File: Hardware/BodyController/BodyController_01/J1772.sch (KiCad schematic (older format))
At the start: 14 parts, among them Q3 2N7002

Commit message: New bring-up code for Body Controller
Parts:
- D9: MPN PMEG10010ELRX -> PMEG6020AELRX
- R177: value 340k -> 560k; MPN ERJ-3EKF3403V -> AC0603FR-07560KL
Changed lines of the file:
@@
 F 1 "D_Schottky" H 2650 1500 50  0000 C CNN
 F 2 "Diodes_SMD:D_SOD-123" H 2650 1600 50  0001 C CNN
-F 3 "https://assets.nexperia.com/documents/data-sheet/PMEG10010ELR.pdf" H 2650 1600 50  0001 C CNN
-F 4 "PMEG10010ELRX" H 2650 1800 50  0001 C CNN "MPN"
+F 3 "https://assets.nexperia.com/documents/data-sheet/PMEG6020AELR.pdf" H 2650 1600 50  0001 C CNN
+F 4 "PMEG6020AELRX" H 2650 1800 50  0001 C CNN "MPN"
 F 5 "y" H 2650 1800 50  0001 C CNN "populate"
 	1    2650 1600
@@
 P 4500 1850
 F 0 "R177" V 4580 1850 50  0000 C CNN
-F 1 "340k" V 4500 1850 50  0000 C CNN
+F 1 "560k" V 4500 1850 50  0000 C CNN
 F 2 "Resistors_SMD:R_0603" V 4430 1850 50  0001 C CNN
-F 3 "https://industrial.panasonic.com/cdbs/www-data/pdf/RDA0000/AOA0000C304.pdf" H 4500 1850 50  0001 C CNN
-F 4 "ERJ-3EKF3403V" H 4580 1950 50  0001 C CNN "MPN"
+F 3 "http://www.yageo.com/NewPortal/yageodocoutput?fileName=/pdf/R-Chip/PYu-AC_51_RoHS_L_6.pdf" H 4500 1850 50  0001 C CNN
+F 4 "AC0603FR-07560KL" H 4580 1950 50  0001 C CNN "MPN"
 F 5 "y" H 4580 1950 50  0001 C CNN "populate"
 	1    4500 1850
@@
 	0    1    1    0
 $EndComp
+$Comp
+L C C138
+U 1 1 5A63943B
+P 2050 1850
+F 0 "C138" H 2075 1950 50  0000 L CNN
+F 1 "10nF" H 2075 1750 50  0000 L CNN
+F 2 "Capacitors_SMD:C_0603" H 2088 1700 50  0001 C CNN
+F 3 "https://product.tdk.com/info/en/documents/chara_sheet/CGA3E2X7R1H103K080AA.pdf" H 2050 1850 50  0001 C CNN
+F 4 "CGA3E2X7R1H103K080AA" H 2075 2050 50  0001 C CNN "MPN"
+F 5 "y" H 2075 2050 50  0001 C CNN "populate"
+	1    2050 1850
+	1    0    0    -1
+$EndComp
+$Comp
+L GND #PWR0284
+U 1 1 5A639442
+P 2050 2050
+F 0 "#PWR0284" H 2050 1800 50  0001 C CNN
+F 1 "GND" H 2050 1900 50  0000 C CNN
+F 2 "" H 2050 2050 50  0001 C CNN
+F 3 "" H 2050 2050 50  0001 C CNN
+	1    2050 2050
+	1    0    0    -1
+$EndComp
+$Comp
+L C C139
+U 1 1 5A6394A0
+P 3650 4650
+F 0 "C139" H 3675 4750 50  0000 L CNN
+F 1 "10nF" H 3675 4550 50  0000 L CNN
+F 2 "Capacitors_SMD:C_0603" H 3688 4500 50  0001 C CNN
+F 3 "https://product.tdk.com/info/en/documents/chara_sheet/CGA3E2X7R1H103K080AA.pdf" H 3650 4650 50  0001 C CNN
+F 4 "CGA3E2X7R1H103K080AA" H 3675 4850 50  0001 C CNN "MPN"
+F 5 "y" H 3675 4850 50  0001 C CNN "populate"
+	1    3650 4650
+	1    0    0    -1
+$EndComp
+$Comp
+L GND #PWR0285
+U 1 1 5A6394A7
+P 3650 4850
+F 0 "#PWR0285" H 3650 4600 50  0001 C CNN
+F 1 "GND" H 3650 4700 50  0000 C CNN
+F 2 "" H 3650 4850 50  0001 C CNN
+F 3 "" H 3650 4850 50  0001 C CNN
+	1    3650 4850
+	1    0    0    -1
+$EndComp
 Text GLabel 1750 1600 0    60   Input ~ 0
 PILOT
@@
 Wire Wire Line
 	3300 4300 4500 4300
+Wire Wire Line
+	2050 2050 2050 2000
+Wire Wire Line
+	3650 4850 3650 4800
+Wire Wire Line
+	2050 1700 2050 1600
+Wire Wire Line
+	3650 4500 3650 4300
 Connection ~ 3200 1600
 Connection ~ 3800 1600
@@
 Connection ~ 5550 4350
 Connection ~ 4500 4300
-$Comp
-L C C138
-U 1 1 5A63943B
-P 2050 1850
-F 0 "C138" H 2075 1950 50  0000 L CNN
-F 1 "10nF" H 2075 1750 50  0000 L CNN
-F 2 "Capacitors_SMD:C_0603" H 2088 1700 50  0001 C CNN
-F 3 "https://product.tdk.com/info/en/documents/chara_sheet/CGA3E2X7R1H103K080AA.pdf" H 2050 1850 50  0001 C CNN
-F 4 "CGA3E2X7R1H103K080AA" H 2075 2050 50  0001 C CNN "MPN"
-F 5 "y" H 2075 2050 50  0001 C CNN "populate"
-	1    2050 1850
-	1    0    0    -1
-$EndComp
-$Comp
-L GND #PWR0284
-U 1 1 5A639442
-P 2050 2050
-F 0 "#PWR0284" H 2050 1800 50  0001 C CNN
-F 1 "GND" H 2050 1900 50  0000 C CNN
-F 2 "" H 2050 2050 50  0001 C CNN
-F 3 "" H 2050 2050 50  0001 C CNN
-	1    2050 2050
-	1    0    0    -1
-$EndComp
-Wire Wire Line
-	2050 2050 2050 2000
-$Comp
-L C C139
-U 1 1 5A6394A0
-P 3650 4650
-F 0 "C139" H 3675 4750 50  0000 L CNN
-F 1 "10nF" H 3675 4550 50  0000 L CNN
-F 2 "Capacitors_SMD:C_0603" H 3688 4500 50  0001 C CNN
-F 3 "https://product.tdk.com/info/en/documents/chara_sheet/CGA3E2X7R1H103K080AA.pdf" H 3650 4650 50  0001 C CNN
-F 4 "CGA3E2X7R1H103K080AA" H 3675 4850 50  0001 C CNN "MPN"
-F 5 "y" H 3675 4850 50  0001 C CNN "populate"
-	1    3650 4650
-	1    0    0    -1
-$EndComp
-$Comp
-L GND #PWR0285
-U 1 1 5A6394A7
-P 3650 4850
-F 0 "#PWR0285" H 3650 4600 50  0001 C CNN
-F 1 "GND" H 3650 4700 50  0000 C CNN
-F 2 "" H 3650 4850 50  0001 C CNN
-F 3 "" H 3650 4850 50  0001 C CNN
-	1    3650 4850
-	1    0    0    -1
-$EndComp
-Wire Wire Line
-	3650 4850 3650 4800
-Wire Wire Line
-	2050 1700 2050 1600
 Connection ~ 2050 1600
-Wire Wire Line
-	3650 4500 3650 4300
 Connection ~ 3650 4300
 $EndSCHEMATC

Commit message: too much work to specify all. New Scheduler, new bootloader, added new Hardware projects, updated code for bringup, COnverted kicad files to new version.
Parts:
- C131, C132, C138, C139: symbol C -> BodyController_01-rescue:C-RESCUE-BodyController_01
- D9: symbol D_Schottky -> BodyController_01-rescue:D_Schottky-RESCUE-BodyController_01
- Q3: symbol 2N7002 -> BodyController_01-rescue:2N7002-RESCUE-BodyController_01
- R176, R177, R178, R179, R180, R181, R73, R82: symbol R -> BodyController_01-rescue:R-RESCUE-BodyController_01
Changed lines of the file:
@@
-EESchema Schematic File Version 2
-LIBS:switches
-LIBS:power
-LIBS:device
-LIBS:transistors
-LIBS:conn
-LIBS:linear
-LIBS:regul
-LIBS:74xx
-LIBS:cmos4000
-LIBS:adc-dac
-LIBS:memory
-LIBS:xilinx
-LIBS:microcontrollers
-LIBS:dsp
-LIBS:microchip
-LIBS:analog_switches
-LIBS:motorola
-LIBS:texas
-LIBS:intel
-LIBS:audio
-LIBS:interface
-LIBS:digital-audio
-LIBS:philips
-LIBS:display
-LIBS:cypress
-LIBS:siliconi
-LIBS:opto
-LIBS:atmel
-LIBS:contrib
-LIBS:valves
-LIBS:HSD
-LIBS:micros
-LIBS:ICs
-LIBS:Connectors
-LIBS:microchip_dspic33dsc
+EESchema Schematic File Version 4
 LIBS:BodyController_01-cache
-EELAYER 25 0
+EELAYER 26 0
 EELAYER END
 $Descr A4 11693 8268
@@
 $EndDescr
 $Comp
-L D_Schottky D9
+L BodyController_01-rescue:D_Schottky-RESCUE-BodyController_01 D9
 U 1 1 5A54F2A1
 P 2650 1600
@@
 $EndComp
 $Comp
-L R R73
+L BodyController_01-rescue:R-RESCUE-BodyController_01 R73
 U 1 1 5A54F30A
 P 3200 1950
@@
 $EndComp
 $Comp
-L R R176
+L BodyController_01-rescue:R-RESCUE-BodyController_01 R176
 U 1 1 5A54F35D
 P 3800 1950
@@
 $EndComp
 $Comp
-L R R177
+L BodyController_01-rescue:R-RESCUE-BodyController_01 R177
 U 1 1 5A54F390
 P 4500 1850
@@
 $EndComp
 $Comp
-L R R178
+L BodyController_01-rescue:R-RESCUE-BodyController_01 R178
 U 1 1 5A54F3DC
 P 4500 2250
@@
 $EndComp
 $Comp
-L GND #PWR0279
+L BodyController_01-rescue:GND-RESCUE-BodyController_01 #PWR0279
 U 1 1 5A54F42F
 P 4500 2550
@@
 $EndComp
 $Comp
-L GND #PWR0280
+L BodyController_01-rescue:GND-RESCUE-BodyController_01 #PWR0280
 U 1 1 5A54F450
 P 3200 2250
@@
 $EndComp
 $Comp
-L C C131
+L BodyController_01-rescue:C-RESCUE-BodyController_01 C131
 U 1 1 5A54F538
 P 4900 2250
@@
 $EndComp
 $Comp
-L 2N7002 Q3
+L BodyController_01-rescue:2N7002-RESCUE-BodyController_01 Q3
 U 1 1 5A54FBF6
 P 3700 2700
@@
 $EndComp
 $Comp
-L GND #PWR0281
+L BodyController_01-rescue:GND-RESCUE-BodyController_01 #PWR0281
 U 1 1 5A54FC4E
 P 3800 3000
@@
 $EndComp
 $Comp
-L R R82
+L BodyController_01-rescue:R-RESCUE-BodyController_01 R82
 U 1 1 5A54FC87
 P 3250 2700
@@
 $EndComp
 $Comp
-L R R179
+L BodyController_01-rescue:R-RESCUE-BodyController_01 R179
 U 1 1 5A54FFEC
 P 4500 4050
@@
 $EndComp
 $Comp
-L R R180
+L BodyController_01-rescue:R-RESCUE-BodyController_01 R180
 U 1 1 5A54FFF2
 P 4500 4550
@@
 $EndComp
 $Comp
-L GND #PWR0282
+L BodyController_01-rescue:GND-RESCUE-BodyController_01 #PWR0282
 U 1 1 5A54FFF8
 P 4500 4850
@@
 $EndComp
 $Comp
-L C C132
+L BodyController_01-rescue:C-RESCUE-BodyController_01 C132
 U 1 1 5A550002
 P 5550 4550
@@
 $EndComp
 $Comp
-L +5VP #PWR0283
+L BodyController_01-rescue:+5VP-RESCUE-BodyController_01 #PWR0283
 U 1 1 5A5505E6
 P 4500 3800
@@
 $EndComp
 $Comp
-L R R181
+L BodyController_01-rescue:R-RESCUE-BodyController_01 R181
 U 1 1 5A5506C3
 P 5150 4350
@@
 $EndComp
 $Comp
-L C C138
+L BodyController_01-rescue:C-RESCUE-BodyController_01 C138
 U 1 1 5A63943B
 P 2050 1850
@@
 $EndComp
 $Comp
-L GND #PWR0284
+L BodyController_01-rescue:GND-RESCUE-BodyController_01 #PWR0284
 U 1 1 5A639442
 P 2050 2050
@@
 $EndComp
 $Comp
-L C C139
+L BodyController_01-rescue:C-RESCUE-BodyController_01 C139
 U 1 1 5A6394A0
 P 3650 4650
@@
 $EndComp
 $Comp
-L GND #PWR0285
+L BodyController_01-rescue:GND-RESCUE-BodyController_01 #PWR0285
 U 1 1 5A6394A7
 P 3650 4850

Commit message: changed some directory locations, added new DCDC PBC project, few Body controller light and switches changes
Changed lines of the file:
@@
 PROXIMITY
 Wire Wire Line
-	2800 1600 4500 1600
+	2800 1600 3200 1600
 Wire Wire Line
 	3200 1600 3200 1800
@@
 	4500 1600 4500 1700
 Wire Wire Line
-	4500 2000 4500 2100
+	4500 2000 4500 2050
 Wire Wire Line
-	4500 2400 4500 2550
+	4500 2400 4500 2450
 Wire Wire Line
 	4900 2100 4900 2050
 Wire Wire Line
-	4500 2050 5150 2050
+	4500 2050 4900 2050
 Wire Wire Line
 	4500 2450 4900 2450
@@
 	3500 2700 3400 2700
 Wire Wire Line
-	1750 1600 2500 1600
+	1750 1600 2050 1600
 Wire Wire Line
 	3100 2700 2900 2700
@@
 	4500 3800 4500 3900
 Wire Wire Line
-	4500 4200 4500 4400
+	4500 4200 4500 4300
 Wire Wire Line
-	4500 4700 4500 4850
+	4500 4700 4500 4750
 Wire Wire Line
 	5550 4400 5550 4350
 Wire Wire Line
-	5300 4350 5800 4350
+	5300 4350 5550 4350
 Wire Wire Line
 	4500 4750 5550 4750
@@
 	5000 4350 4500 4350
 Wire Wire Line
-	3300 4300 4500 4300
+	3300 4300 3650 4300
 Wire Wire Line
 	2050 2050 2050 2000
@@
 Connection ~ 2050 1600
 Connection ~ 3650 4300
+Wire Wire Line
+	3200 1600 3800 1600
+Wire Wire Line
+	3800 1600 4500 1600
+Wire Wire Line
+	4500 2050 4500 2100
+Wire Wire Line
+	4500 2450 4500 2550
+Wire Wire Line
+	4900 2050 5150 2050
+Wire Wire Line
+	4500 4350 4500 4400
+Wire Wire Line
+	4500 4750 4500 4850
+Wire Wire Line
+	5550 4350 5800 4350
+Wire Wire Line
+	4500 4300 4500 4350
+Wire Wire Line
+	2050 1600 2500 1600
+Wire Wire Line
+	3650 4300 4500 4300
 $EndSCHEMATC

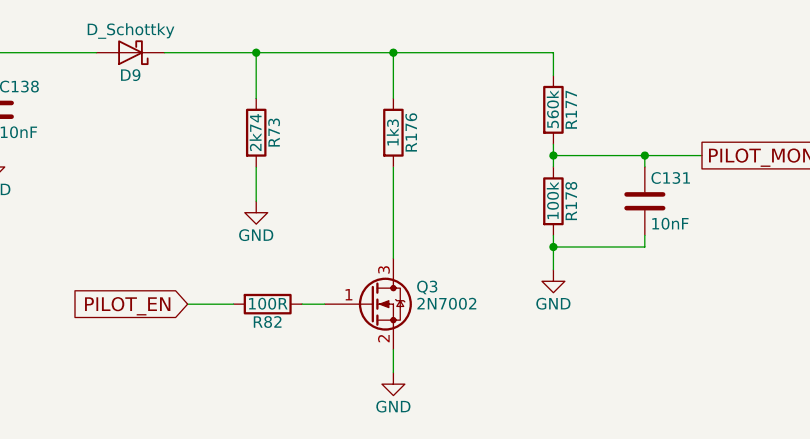
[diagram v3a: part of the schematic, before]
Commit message: Too much stuff to list
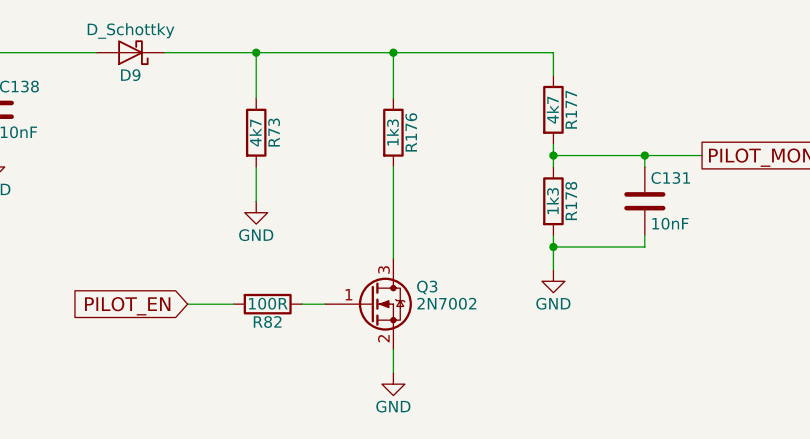
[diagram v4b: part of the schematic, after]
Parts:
- R177: value 560k -> 4k7; MPN AC0603FR-07560KL -> (none)
- R178: value 100k -> 1k3; MPN AC0603FR-07100KL -> (none)
- R73: value 2k74 -> 4k7; MPN AC0603FR-072K74L -> (none)
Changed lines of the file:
@@
 P 3200 1950
 F 0 "R73" V 3280 1950 50  0000 C CNN
-F 1 "2k74" V 3200 1950 50  0000 C CNN
+F 1 "4k7" V 3200 1950 50  0000 C CNN
 F 2 "Resistors_SMD:R_0603" V 3130 1950 50  0001 C CNN
-F 3 "http://www.yageo.com/NewPortal/yageodocoutput?fileName=/pdf/R-Chip/PYu-AC_51_RoHS_L_6.pdf" H 3200 1950 50  0001 C CNN
-F 4 "AC0603FR-072K74L" H 3280 2050 50  0001 C CNN "MPN"
+F 3 "fileName=/pdf/R-Chip/PYu-AC_51_RoHS_L_6.pdf" H 3200 1950 50  0001 C CNN
+F 4 "~" H 3280 2050 50  0001 C CNN "MPN"
 F 5 "y" H 3280 2050 50  0001 C CNN "populate"
 	1    3200 1950
@@
 P 4500 1850
 F 0 "R177" V 4580 1850 50  0000 C CNN
-F 1 "560k" V 4500 1850 50  0000 C CNN
+F 1 "4k7" V 4500 1850 50  0000 C CNN
 F 2 "Resistors_SMD:R_0603" V 4430 1850 50  0001 C CNN
-F 3 "http://www.yageo.com/NewPortal/yageodocoutput?fileName=/pdf/R-Chip/PYu-AC_51_RoHS_L_6.pdf" H 4500 1850 50  0001 C CNN
-F 4 "AC0603FR-07560KL" H 4580 1950 50  0001 C CNN "MPN"
+F 3 "fileName=/pdf/R-Chip/PYu-AC_51_RoHS_L_6.pdf" H 4500 1850 50  0001 C CNN
+F 4 "~" H 4580 1950 50  0001 C CNN "MPN"
 F 5 "y" H 4580 1950 50  0001 C CNN "populate"
 	1    4500 1850
@@
 P 4500 2250
 F 0 "R178" V 4580 2250 50  0000 C CNN
-F 1 "100k" V 4500 2250 50  0000 C CNN
+F 1 "1k3" V 4500 2250 50  0000 C CNN
 F 2 "Resistors_SMD:R_0603" V 4430 2250 50  0001 C CNN
-F 3 "http://www.yageo.com/NewPortal/yageodocoutput?fileName=/pdf/R-Chip/PYu-AC_51_RoHS_L_6.pdf" H 4500 2250 50  0001 C CNN
-F 4 "AC0603FR-07100KL" H 4580 2350 50  0001 C CNN "MPN"
+F 3 "" H 4500 2250 50  0001 C CNN
+F 4 "~" H 4580 2350 50  0001 C CNN "MPN"
 F 5 "y" H 4580 2350 50  0001 C CNN "populate"
 	1    4500 2250
@@
 F 5 "y" H 4580 4150 50  0001 C CNN "populate"
 	1    4500 4050
-	1    0    0    -1
-$EndComp
-$Comp
-L BodyController_01-rescue:R-RESCUE-BodyController_01 R180
-U 1 1 5A54FFF2
-P 4500 4550
-F 0 "R180" V 4580 4550 50  0000 C CNN
-F 1 "330R" V 4500 4550 50  0000 C CNN
-F 2 "Resistors_SMD:R_0603" V 4430 4550 50  0001 C CNN
-F 3 "http://www.yageo.com/NewPortal/yageodocoutput?fileName=/pdf/R-Chip/PYu-AC_51_RoHS_L_6.pdf" H 4500 4550 50  0001 C CNN
-F 4 "AC0603FR-07330RL" H 4580 4650 50  0001 C CNN "MPN"
-F 5 "y" H 4580 4650 50  0001 C CNN "populate"
-	1    4500 4550
 	1    0    0    -1
 $EndComp
@@
 Wire Wire Line
 	3650 4300 4500 4300
+$Comp
+L BodyController_01-rescue:R-RESCUE-BodyController_01 R180
+U 1 1 5D1A16D4
+P 4500 4550
+F 0 "R180" V 4580 4550 50  0000 C CNN
+F 1 "330R" V 4500 4550 50  0000 C CNN
+F 2 "Resistors_SMD:R_0603" V 4430 4550 50  0001 C CNN
+F 3 "http://www.yageo.com/NewPortal/yageodocoutput?fileName=/pdf/R-Chip/PYu-AC_51_RoHS_L_6.pdf" H 4500 4550 50  0001 C CNN
+F 4 "AC0603FR-07330RL" H 4580 4650 50  0001 C CNN "MPN"
+F 5 "y" H 4580 4650 50  0001 C CNN "populate"
+	1    4500 4550
+	1    0    0    -1
+$EndComp
 $EndSCHEMATC
